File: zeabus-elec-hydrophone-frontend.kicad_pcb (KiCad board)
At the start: 4 copper layers, 53.3 x 68.6 mm, 153 parts, among them CN1 EPS.00.250.NTN, CN2 EPS.00.250.NTN, CN3 EPS.00.250.NTN, CN4 EPS.00.250.NTN, J1 Conn_R1, J10 TEST_1P, J11 TEST_1P, J12 TEST_1P, J13 TEST_1P, J14 TEST_1P, J15 TEST_1P, J16 TEST_1P, J17 TEST_1P, J18 TEST_1P, J2 Conn_L1, J3 Conn_R2, J4 Conn_L2, J5 TEST_1P, J6 TEST_1P, J7 TEST_1P, J8 TEST_1P, J9 TEST_1P, U1 AD8334ACPZ, U2 TLV73311PDBVT, U3 MAX5387LAUD+T, U4 OPA2365, U5 OPA2365

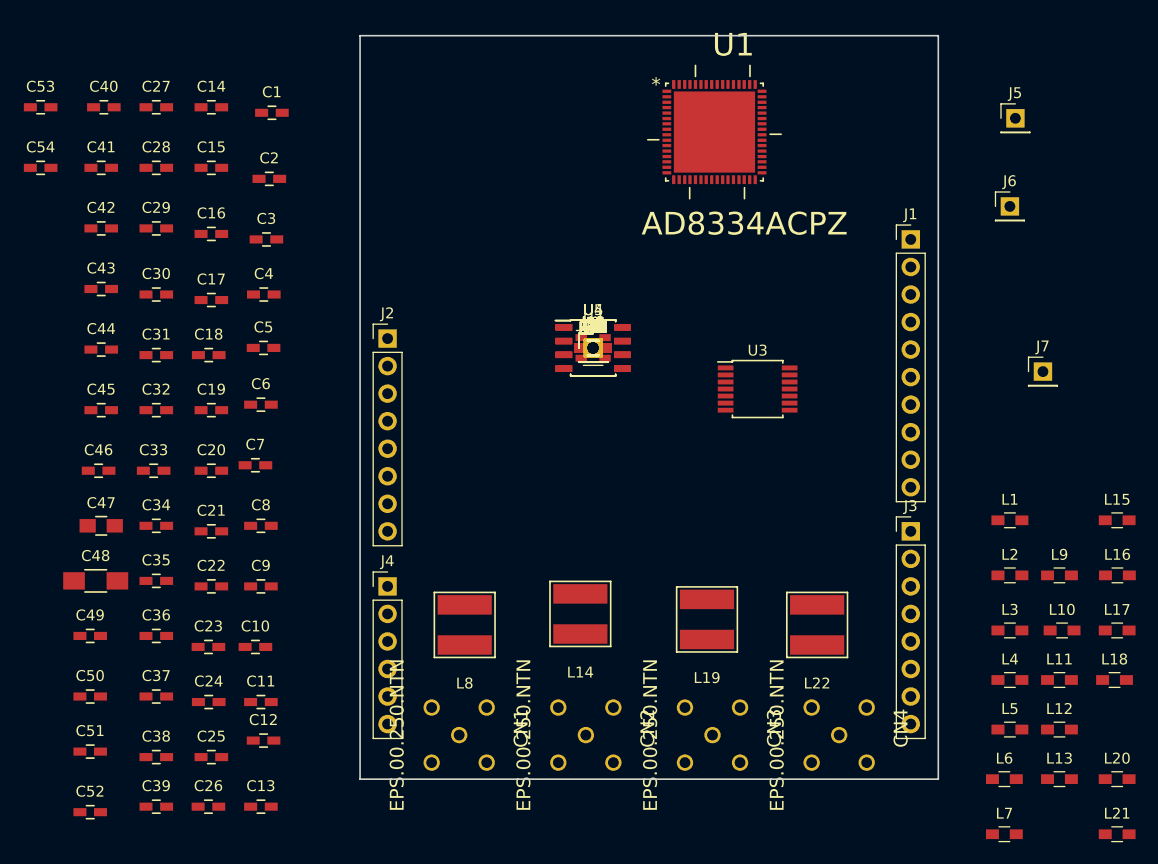
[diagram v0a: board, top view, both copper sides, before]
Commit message: First released
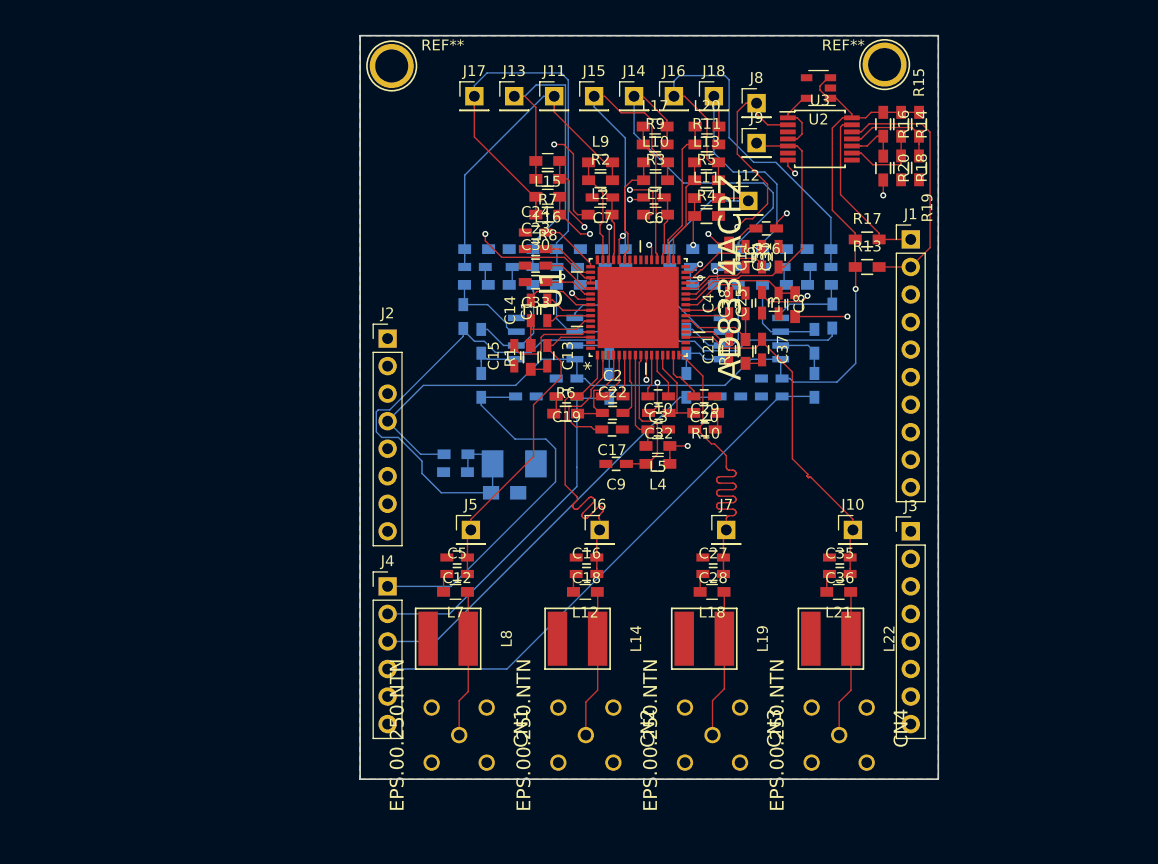
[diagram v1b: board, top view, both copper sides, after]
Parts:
- added REF**: 1pin, Connectors:1pin, F.Cu at (175.4, 78.9)
- added REF**: 1pin, Connectors:1pin, F.Cu at (129.9, 79.0)
- C39, C40, C41, C42, C43, C44, C45, C46, C47, C49, C50, C51, C52, C53, C54, R21, R22, R23, R24, R25, R26, R27, R28, R29, R30, R31, R32, R33, R34, R35, R36, R37, R38, R39, R40, R41, R42, R43, R44, R45, R46, R47, R48, R49, R50, U4, U5: moved to B.Cu
- C48: footprint Capacitors_SMD:C_1206_HandSoldering -> Capacitors_SMD:C_1210_HandSoldering; moved to B.Cu
- moved C50 78.2 mm to (169.5, 97.5), turned to 180 degrees
- moved C26 74.1 mm to (164.5, 94.0), turned to 180 degrees
- moved C52 73.6 mm to (165.0, 109.5), turned to 180 degrees
- moved L20 71.1 mm to (159.0, 84.6)
- moved C38 68.6 mm to (162.6, 100.9), turned to 90 degrees
- moved C54 68.2 mm to (165.2, 97.5)
- moved C27 67.0 mm to (159.6, 125.9)
- moved C25 65.9 mm to (164.1, 100.8), turned to 90 degrees
- moved L13 65.6 mm to (159.0, 87.9)
- moved C37 64.4 mm to (164.1, 105.2), turned to 270 degrees
- moved C36 63.5 mm to (171.3, 124.3), turned to 180 degrees
- moved C42 63.4 mm to (165.0, 107.8), turned to 180 degrees
- moved L16 63.1 mm to (144.3, 91.1), turned to 180 degrees
- moved L17 63.1 mm to (154.2, 84.6)
- moved C35 63.1 mm to (171.3, 125.9)
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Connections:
- U2 pad 1: +3.3VA -> +3V3
- U2 pad 3: +3.3VA -> +3V3
- U4 pad 5: Net-(R22-Pad1) -> Net-(R37-Pad1)
- U4 pad 6: Net-(R32-Pad1) -> Net-(R47-Pad1)
- U4 pad 7: Net-(R28-Pad2) -> Net-(R43-Pad2)
- U5 pad 1: Net-(R43-Pad2) -> Net-(R28-Pad2)
- U5 pad 2: Net-(R47-Pad1) -> Net-(R32-Pad1)
- U5 pad 3: Net-(R37-Pad1) -> Net-(R22-Pad1)
- U5 pad 4: Net-(U5-Pad4) -> GNDA
- U5 pad 8: Net-(U5-Pad8) -> +3V3
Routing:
- net +3V3: track 0.00 -> 94.6 mm, vias 0 -> 1
- net VA_REF: track 0.00 -> 72.8 mm
- net /ADC3: track 0.00 -> 49.8 mm
- net +5V: track 0.00 -> 43.0 mm, vias 0 -> 7
- net /LNA Gain Control/GAIN12: track 0.00 -> 42.8 mm, vias 0 -> 2
- net /LNA/LNA1RN: track 0.00 -> 41.5 mm
- net /ADC2: track 0.00 -> 40.0 mm
- net /LNA/LNA2RP: track 0.00 -> 39.7 mm
- net /ADC0: track 0.00 -> 35.0 mm
- net /ADC1: track 0.00 -> 33.7 mm
- net /LNA/INH3: track 0.00 -> 33.5 mm
- net /LNA/INH4: track 0.00 -> 33.1 mm
- net /LNA/LNA2LN: track 0.00 -> 32.9 mm
- net /LNA/LNA1LN: track 0.00 -> 32.2 mm
- net /LNA/LNA1LP: track 0.00 -> 30.1 mm
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- added copper zone on In2.Cu, net +5V
- added copper zone on B.Cu, net GNDA
- added copper zone on F.Cu, net GNDA
- added copper zone on In1.Cu, net GNDA
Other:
- net class Default: clearance 0.2 -> 0.127; trace_width 0.25 -> 0.127; via_dia 0.6 -> 0.5588; via_drill 0.4 -> 0.3048
- rule trace_clearance: 0.2 -> 0.127
- rule trace_min: 0.2 -> 0.127
- rule via_min_drill: 0.3 -> 0.3048
- rule via_min_size: 0.4 -> 0.5588
